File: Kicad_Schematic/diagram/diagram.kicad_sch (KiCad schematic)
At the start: 10 parts, among them U1 Pico

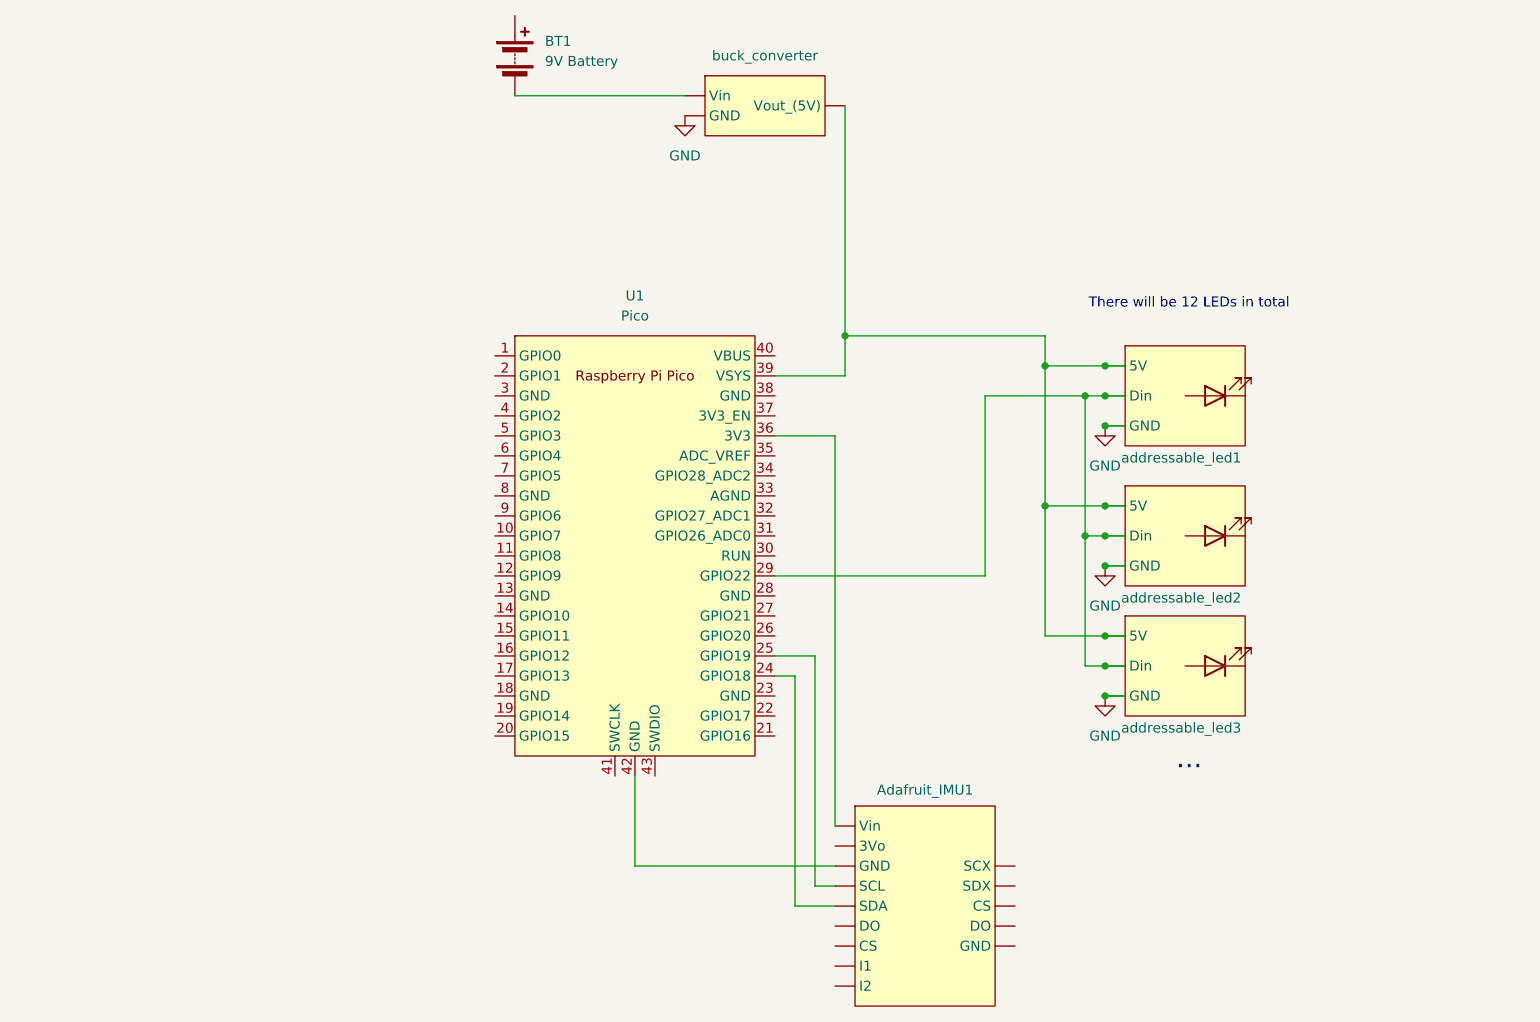
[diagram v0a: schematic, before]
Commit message: Finalized Kicad Schematic
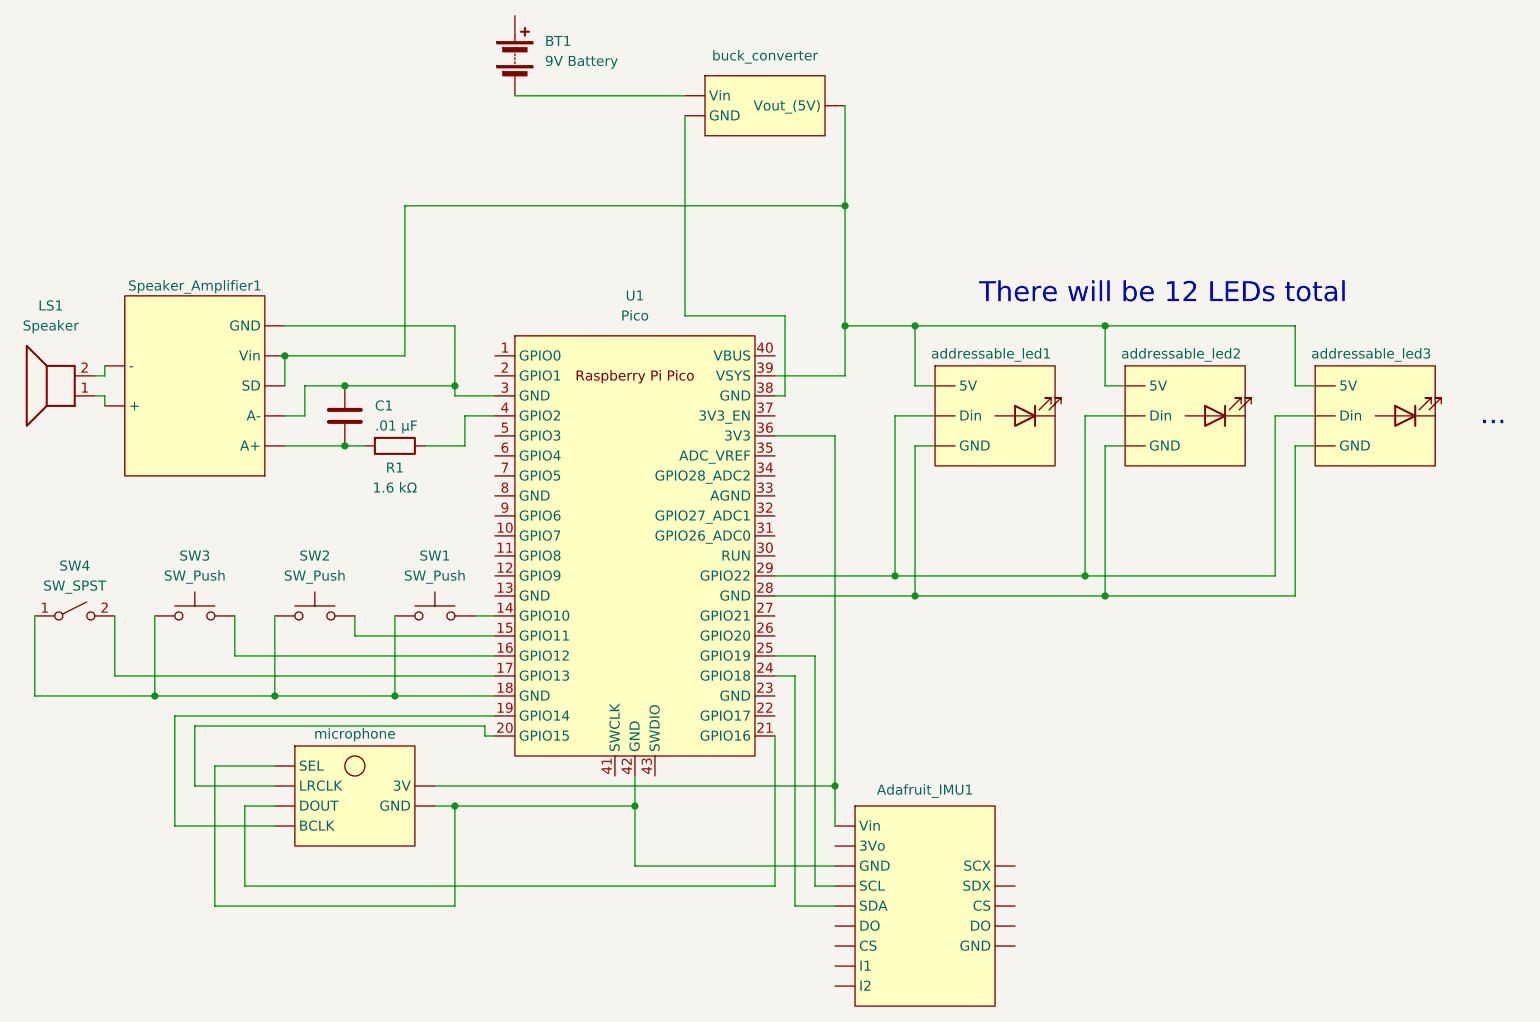
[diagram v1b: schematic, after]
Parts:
- added C1: .01 µF, symbol Device:C
- added LS1: Speaker, symbol Device:Speaker
- added R1: 1.6 kΩ, symbol Device:R
- added SW1, SW2, SW3: SW_Push, symbol Switch:SW_Push
- added SW4: SW_SPST, symbol Switch:SW_SPST
- added Speaker_Amplifier1: ~, symbol New_Library:Speaker_Amplifier
- added microphone: ~, symbol New_Library:microphone
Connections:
- net at addressable_led1. (GND), addressable_led2. (GND), addressable_led3. (GND): now also U1.29 (GPIO22); no longer U1.39 (VSYS), buck_converter. (Vout_(5V))
- net at U1.14 (GPIO10): now also SW1.2
- net at U1.15 (GPIO11): now also SW2.2
- net at U1.16 (GPIO12): now also SW3.2
- net at U1.17 (GPIO13): now also SW4.2 (B)
- net at U1.18 (GND): now also SW1.1, SW2.1, SW3.1, SW4.1 (A)
- net at U1.19 (GPIO14): now also microphone. (GND)
- net at U1.20 (GPIO15): now also microphone. (GND)
- net at U1.21 (GPIO16): now also microphone. (GND)
- net at U1.28 (GND): now also addressable_led1. (GND), addressable_led2. (GND), addressable_led3. (GND)
- net at U1.3 (GND): now also C1.1, Speaker_Amplifier1. (-)
- net at Adafruit_IMU1. (GND), U1.36 (3V3): now also microphone. (GND)
- net at U1.38 (GND): now also buck_converter. (Vout_(5V))
- net at U1.4 (GPIO2): now also R1.1
- net at Adafruit_IMU1. (GND), U1.42 (GND): now also microphone. (GND)
- removed net GND: addressable_led1. (GND), addressable_led2. (GND), addressable_led3. (GND), buck_converter. (Vout_(5V))
- new net: C1.2, R1.2, Speaker_Amplifier1. (-)
- new net: Speaker_Amplifier1. (-), U1.39 (VSYS), addressable_led1. (GND), addressable_led2. (GND), addressable_led3. (GND), buck_converter. (Vout_(5V))
- new net: LS1.1, Speaker_Amplifier1. (-)
- new net: LS1.2, Speaker_Amplifier1. (-)
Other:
- note added: "There will be 12 LEDs total"
- note removed: "There will be 12 LEDs in total"
- title: (none) -> ECE2799 Team 3 Circuit Schematic
